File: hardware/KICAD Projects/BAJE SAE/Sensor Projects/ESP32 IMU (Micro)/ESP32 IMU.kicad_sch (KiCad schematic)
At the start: 6 parts, among them J1 Conn_01x02, J2 CAN to outer connector, J3 Conn_01x06

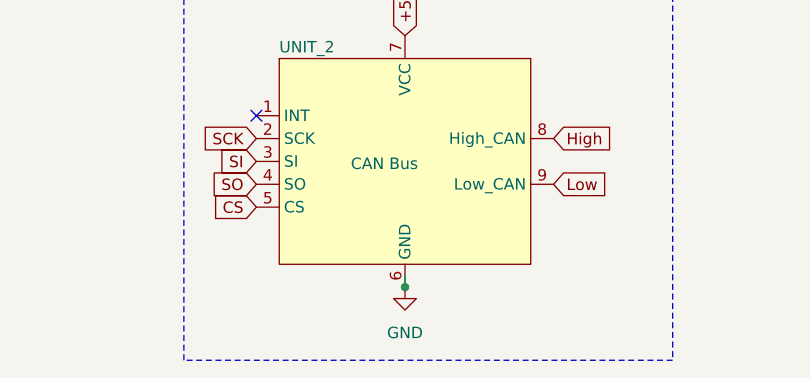
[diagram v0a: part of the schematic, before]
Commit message: finished pcbs yayyyy
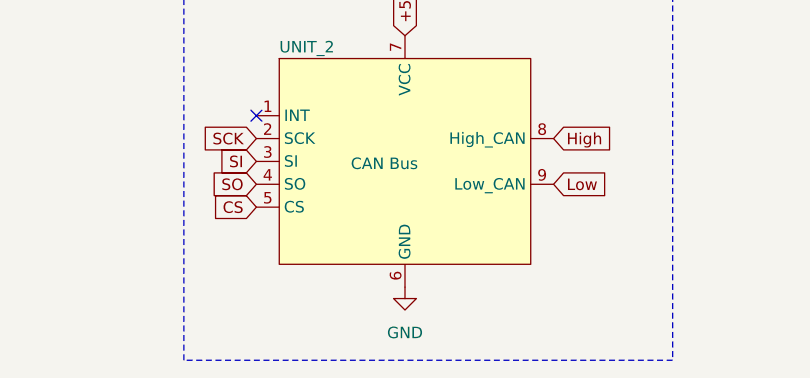
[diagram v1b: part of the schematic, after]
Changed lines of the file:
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@@
 		(comment 1 "Connor Larson")
-	)
-	(junction
-		(at 133.35 190.5)
-		(diameter 0)
-		(color 0 0 0 0)
 	)
 	(no_connect
@@
 		(pts
 			(xy 114.3 96.52) (xy 132.08 96.52)
-		)
-		(stroke
-			(width 0)
-			(type default)
-		)
-	)
-	(wire
-		(pts
-			(xy 133.35 189.23) (xy 133.35 190.5)
 		)
 		(stroke
@@
 		(dnp no)
 		(fields_autoplaced yes)
-		(property "Reference" "#PWR07"
+		(property "Reference" "#PWR02"
 			(at 133.35 196.85 0)
 			(effects
@@
 		)
 		(instances
-			(project ""
+			(project "ESP32 IMU"
 				(path "/7db5226c-054a-443a-bdfe-e8f86c4e465d"
-					(reference "#PWR07")
+					(reference "#PWR02")
 					(unit 1)
 				)

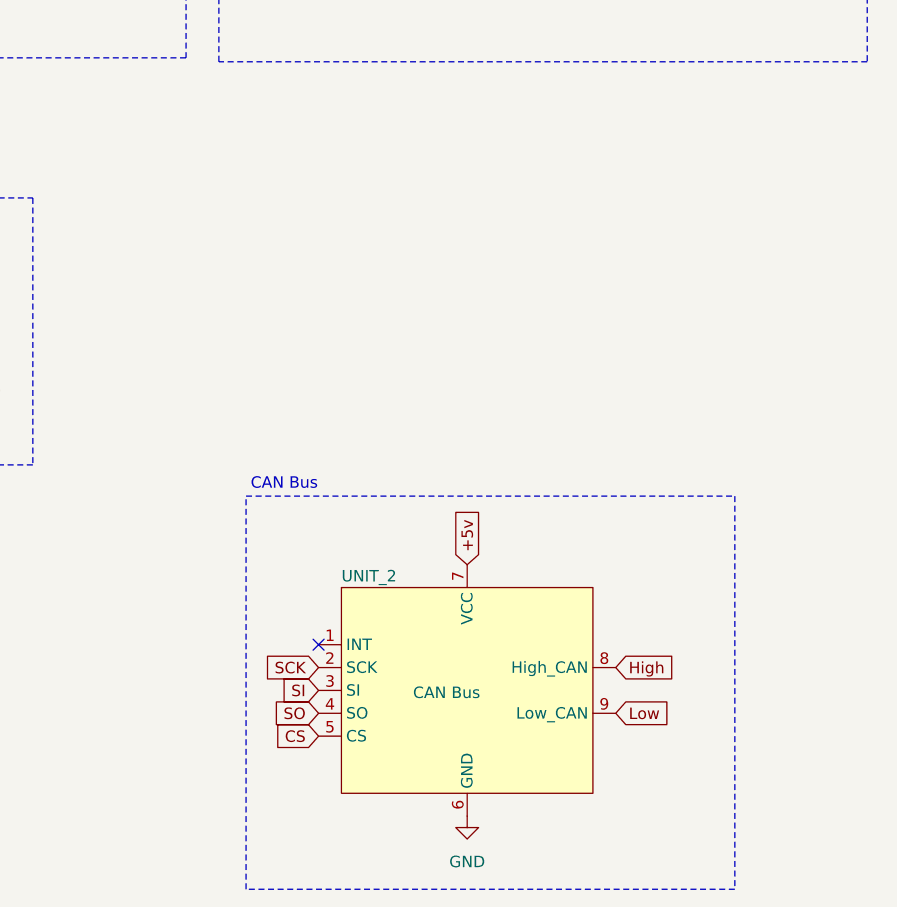
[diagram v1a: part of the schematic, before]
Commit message: dash updates
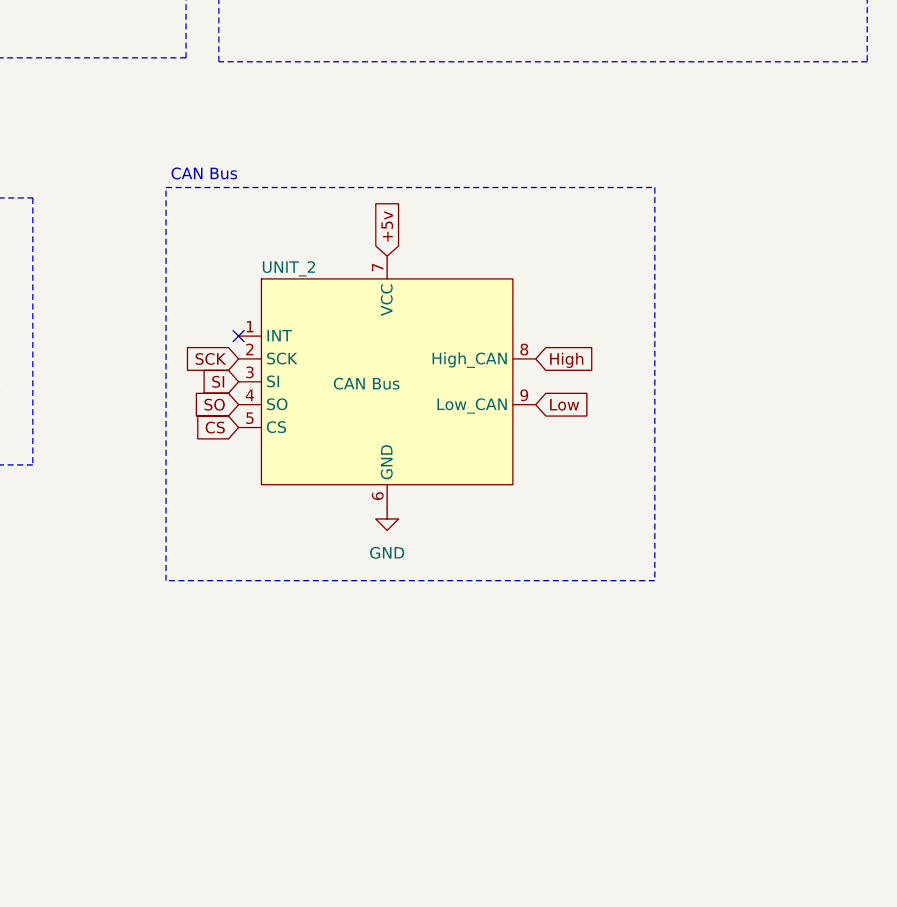
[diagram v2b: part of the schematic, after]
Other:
- moved on the sheet: UNIT_2
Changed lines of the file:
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@@
 	)
 	(no_connect
-		(at 116.84 171.45)
+		(at 107.95 137.16)
 	)
 	(no_connect
@@
 	)
 	(rectangle
-		(start 108.7808 154.94)
-		(end 163.0904 198.6232)
+		(start 99.8908 120.65)
+		(end 154.2004 164.3332)
 		(stroke
 			(width 0)
@@
 	(text "CAN Bus"
 		(exclude_from_sim no)
-		(at 113.03 153.67 0)
+		(at 104.14 119.38 0)
 		(effects
 			(font
@@
 	(global_label "+5v"
 		(shape input)
-		(at 133.35 162.56 90)
+		(at 124.46 128.27 90)
 		(fields_autoplaced yes)
 		(effects
@@
 		)
 		(property "Intersheetrefs" "${INTERSHEET_REFS}"
-			(at 133.35 155.8253 90)
+			(at 124.46 121.5353 90)
 			(effects
 				(font
@@
 	(global_label "SCK"
 		(shape input)
-		(at 116.84 173.99 180)
+		(at 107.95 139.7 180)
 		(fields_autoplaced yes)
 		(effects
@@
 		)
 		(property "Intersheetrefs" "${INTERSHEET_REFS}"
-			(at 110.1053 173.99 0)
+			(at 101.2153 139.7 0)
 			(effects
 				(font
@@
 	(global_label "CS"
 		(shape input)
-		(at 116.84 181.61 180)
+		(at 107.95 147.32 180)
 		(fields_autoplaced yes)
 		(effects
@@
 		)
 		(property "Intersheetrefs" "${INTERSHEET_REFS}"
-			(at 111.3753 181.61 0)
+			(at 102.4853 147.32 0)
 			(effects
 				(font
@@
 	(global_label "SO"
 		(shape input)
-		(at 116.84 179.07 180)
+		(at 107.95 144.78 180)
 		(fields_autoplaced yes)
 		(effects
@@
 		)
 		(property "Intersheetrefs" "${INTERSHEET_REFS}"
-			(at 111.3148 179.07 0)
+			(at 102.4248 144.78 0)
 			(effects
 				(font
@@
 	(global_label "SI"
 		(shape input)
-		(at 116.84 176.53 180)
+		(at 107.95 142.24 180)
 		(fields_autoplaced yes)
 		(effects
@@
 		)
 		(property "Intersheetrefs" "${INTERSHEET_REFS}"
-			(at 112.0405 176.53 0)
+			(at 103.1505 142.24 0)
 			(effects
 				(font
@@
 	(global_label "Low"
 		(shape input)
-		(at 149.86 179.07 0)
+		(at 140.97 144.78 0)
 		(fields_autoplaced yes)
 		(effects
@@
 		)
 		(property "Intersheetrefs" "${INTERSHEET_REFS}"
-			(at 156.3528 179.07 0)
+			(at 147.4628 144.78 0)
 			(effects
 				(font
@@
 	(global_label "High"
 		(shape input)
-		(at 149.86 173.99 0)
+		(at 140.97 139.7 0)
 		(fields_autoplaced yes)
 		(effects
@@
 		)
 		(property "Intersheetrefs" "${INTERSHEET_REFS}"
-			(at 157.0785 173.99 0)
+			(at 148.1885 139.7 0)
 			(effects
 				(font
@@
 	(symbol
 		(lib_id "BAJA SAE:HiLetgo_CAN_BUS")
-		(at 133.35 176.53 0)
+		(at 124.46 142.24 0)
 		(unit 1)
 		(exclude_from_sim no)
@@
 		(dnp no)
 		(property "Reference" "UNIT_2"
-			(at 119.38 163.83 0)
+			(at 110.49 129.54 0)
 			(effects
 				(font
@@
 		)
 		(property "Value" "CAN Bus"
-			(at 131.064 176.784 0)
+			(at 122.174 142.494 0)
 			(effects
 				(font
@@
 		)
 		(property "Footprint" "BAJA SAE:HiLetgo CAN Bus"
-			(at 133.604 197.866 0)
+			(at 124.714 163.576 0)
 			(effects
 				(font
@@
 		)
 		(property "Datasheet" ""
-			(at 129.54 172.72 0)
+			(at 120.65 138.43 0)
 			(effects
 				(font
@@
 		)
 		(property "Description" ""
-			(at 129.54 172.72 0)
+			(at 120.65 138.43 0)
 			(effects
 				(font
@@
 	(symbol
 		(lib_id "power:GND")
-		(at 133.35 190.5 0)
+		(at 124.46 156.21 0)
 		(unit 1)
 		(exclude_from_sim no)
@@
 		(fields_autoplaced yes)
 		(property "Reference" "#PWR02"
-			(at 133.35 196.85 0)
+			(at 124.46 162.56 0)
 			(effects
 				(font
@@
 		)
 		(property "Value" "GND"
-			(at 133.35 195.58 0)
+			(at 124.46 161.29 0)
 			(effects
 				(font
@@
 		)
 		(property "Footprint" ""
-			(at 133.35 190.5 0)
+			(at 124.46 156.21 0)
 			(effects
 				(font
@@
 		)
 		(property "Datasheet" ""
-			(at 133.35 190.5 0)
+			(at 124.46 156.21 0)
 			(effects
 				(font
@@
 		)
 		(property "Description" "Power symbol creates a global label with name \"GND\" , ground"
-			(at 133.35 190.5 0)
-			(effects
-				(font
+			(at 124.46 156.21 0)
+			(effects
+				(font
